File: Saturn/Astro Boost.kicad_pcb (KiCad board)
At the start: 2 copper layers, 56 x 82.2 mm, 35 parts, among them J1 AudioJack2, J10 Power from SW to PS, J11 +9V, J12 -9V, J2 AudioJack2, J3 Jack-DC, J4 Signal In, J5 Audio In, J6 Processed to SW, J7 Bypass, J8 Processed Out, J9 Power from 9V to SW, Q1 OC44, SW1 SW_Nidec_CAS-120A1, U1 MAX1044

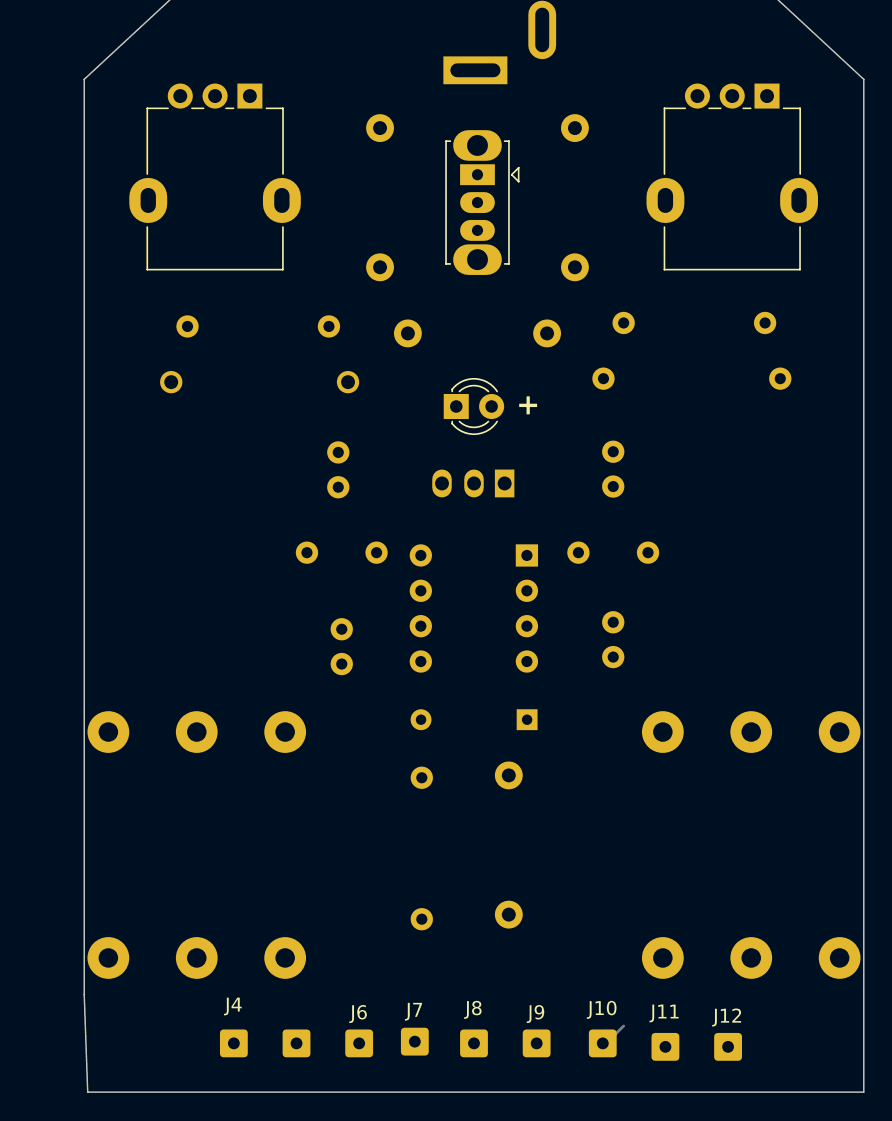
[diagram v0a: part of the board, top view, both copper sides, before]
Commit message: Updates to saturn
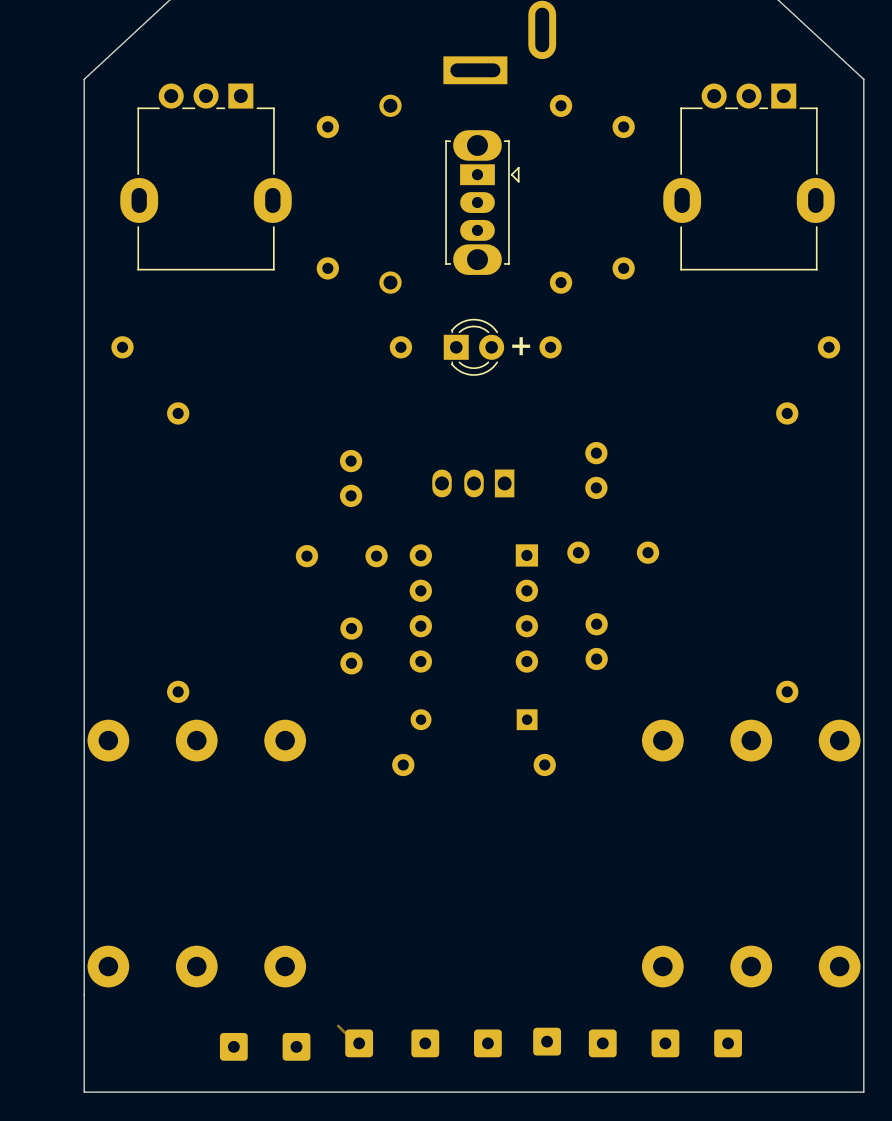
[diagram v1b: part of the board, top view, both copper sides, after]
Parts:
- C1, C5: footprint Capacitor_THT:C_Disc_D9.0mm_W5.0mm_P10.00mm -> Capacitor_THT:C_Axial_L12.0mm_D6.5mm_P20.00mm_Horizontal
- C2, C4: footprint Capacitor_THT:C_Disc_D9.0mm_W5.0mm_P10.00mm -> Capacitor_THT:C_Axial_L12.0mm_D9.5mm_P20.00mm_Horizontal
- J10, J11, J12, J4, J5, J6, J7, J8, J9: moved to B.Cu
- moved C4 42.3 mm to (172.8, 78.5)
- moved J12 35.5 mm to (133.0, 104.0), turned to 180 degrees
- moved J4 35.5 mm to (168.5, 103.8), turned to 180 degrees
- moved C2 35.2 mm to (129.0, 58.5)
- moved J11 26.5 mm to (137.5, 104.0), turned to 180 degrees
- moved J5 26.5 mm to (164.0, 103.8), turned to 180 degrees
- moved C1 24.1 mm to (175.8, 53.8), turned to 180 degrees
- moved C5 20.5 mm to (125.0, 53.8)
- moved J10 17.5 mm to (142.0, 103.8), turned to 180 degrees
- moved J6 17.5 mm to (159.5, 103.8), turned to 180 degrees
- moved R1 17.2 mm to (156.5, 49.1), turned to 90 degrees
- moved R2 11.2 mm to (145.2, 83.8), turned to 0 degrees
- moved R4 10.9 mm to (161.0, 48.1), turned to 90 degrees
- moved J7 9.50 mm to (155.5, 103.6), turned to 180 degrees
- moved J9 8.00 mm to (146.8, 103.8), turned to 180 degrees
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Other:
- outline, holes or cut-outs redrawn
- board text added: "C10"
- board text added: "C2"
- board text added: "C3"
- board text added: "C4"
- board text added: "C6"
- board text added: "C7"
- board text added: "C8"
- board text added: "C9"
- board text added: "D2"
- board text added: "Q1"
- board text added: "R1"
- board text added: "R3"
